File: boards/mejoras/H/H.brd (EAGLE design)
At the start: 100 x 35 mm, 37 parts, among them IC1 PIC18F4455_TQFP

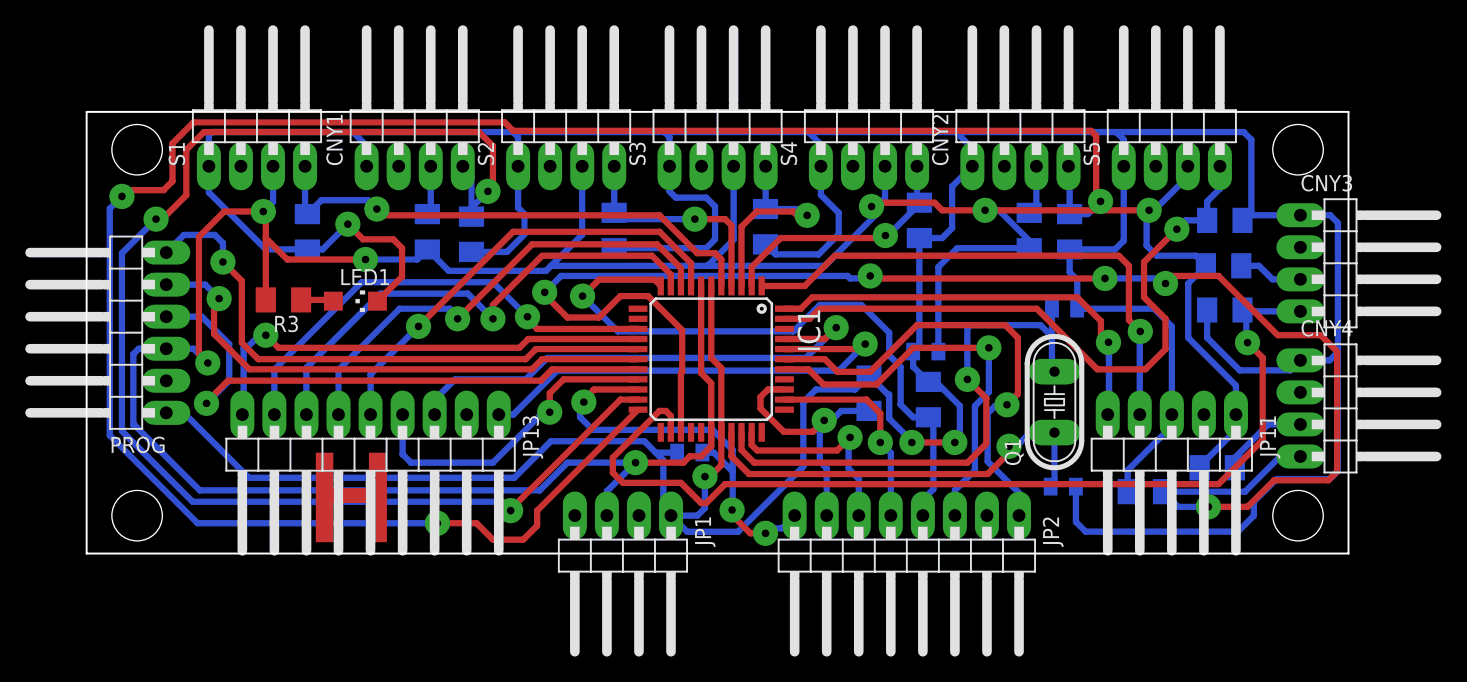
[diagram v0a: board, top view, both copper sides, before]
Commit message: updated board h and i
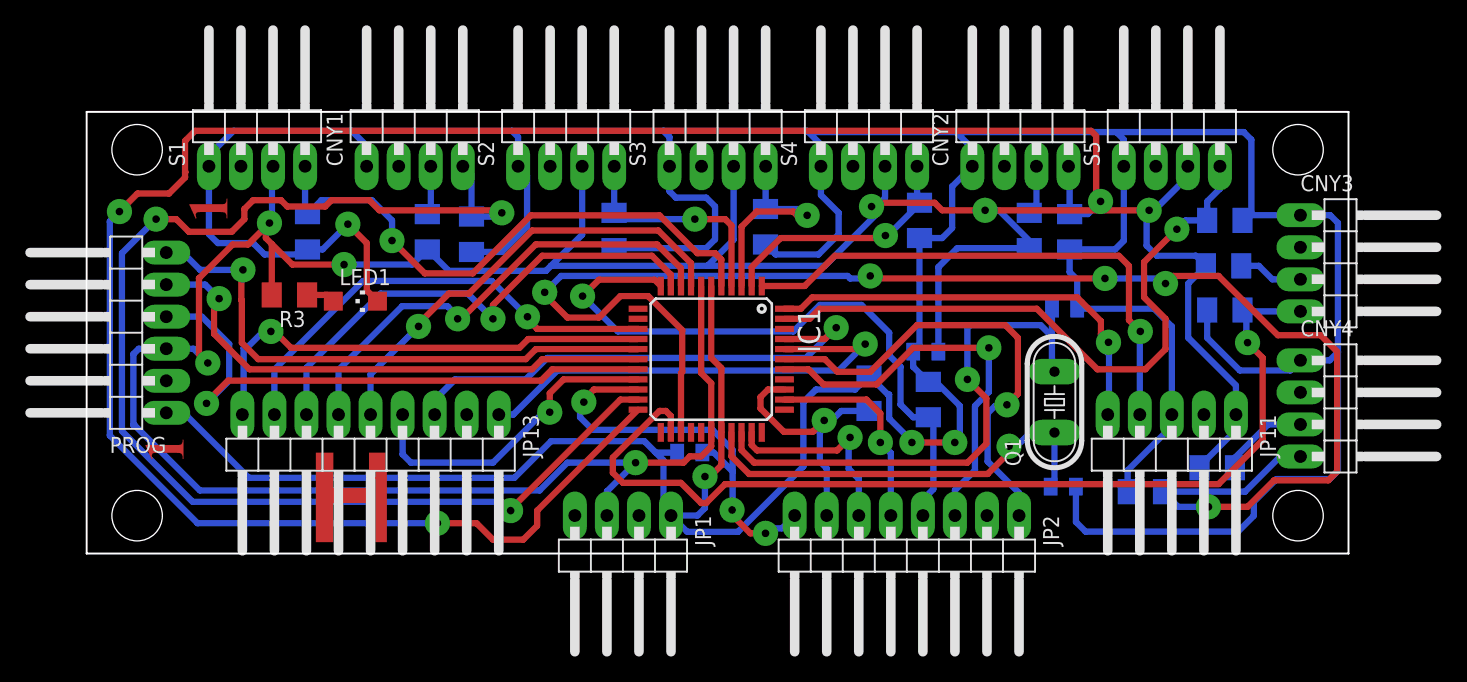
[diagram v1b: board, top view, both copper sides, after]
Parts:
- moved R3 0.61 mm to (16.1, 20.5)
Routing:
- net CNY1: track 107.8 -> 102.1 mm
- net S1: track 41.2 -> 45.9 mm
- net 5V: track 256.8 -> 254.4 mm
- net PGC: track 46.1 -> 44.8 mm
- net CNY2: track 163.5 -> 162.3 mm
- net GND: track 417.6 -> 416.7 mm
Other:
- board text added: "C:/Users/Ariel/GitHub/Sumo-Robot-Programs-Database/boards/mejoras/I/1.bmp"

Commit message: small fixes to h
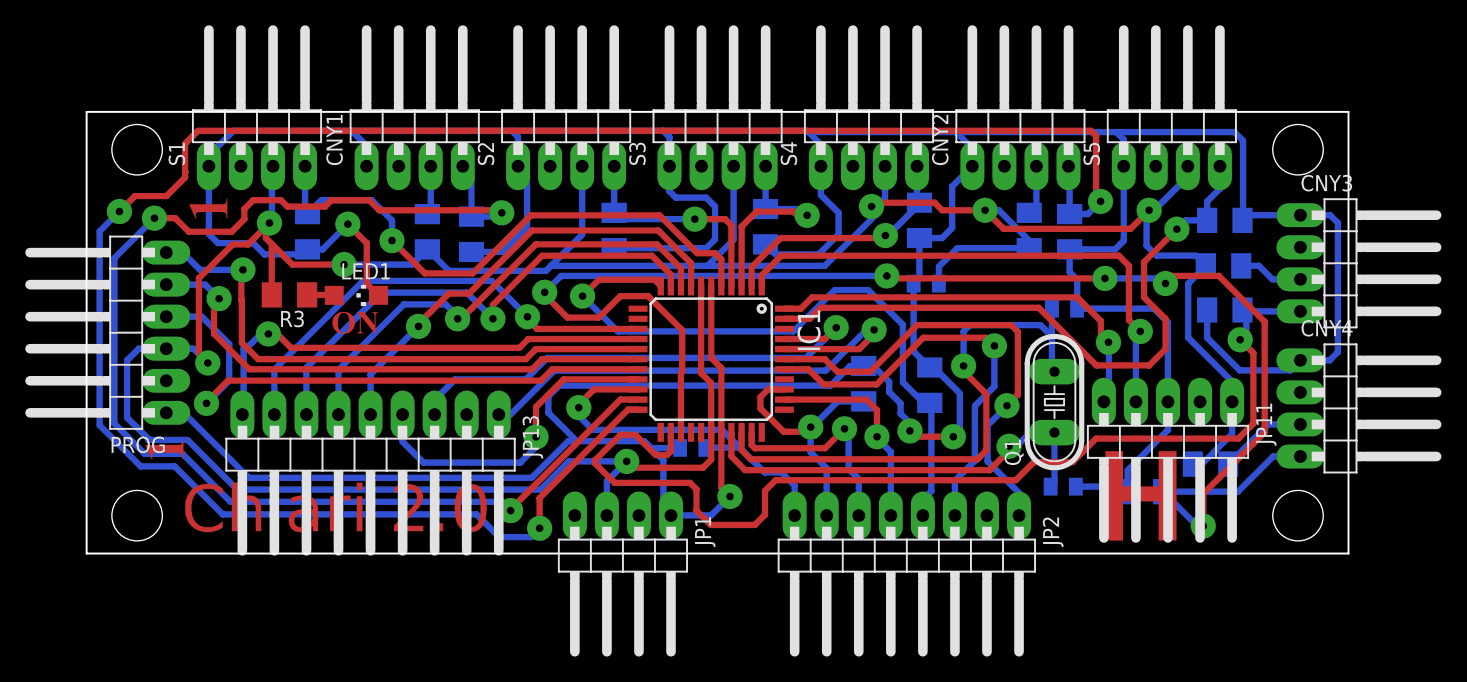
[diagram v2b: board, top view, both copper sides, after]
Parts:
- moved C3 5.39 mm to (66.5, 21.4)
- moved R1 1.15 mm to (66.8, 13.3)
- moved JP11 1.06 mm to (85.7, 8.22)
- moved R2 0.87 mm to (61.6, 13.5)
- moved R16 0.60 mm to (89.1, 7.08)
- moved LED1 0.46 mm to (21.4, 20.5)
- moved C4 0.43 mm to (48.0, 8.36)
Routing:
- net GND: track 416.7 -> 391.0 mm
- net CNY4: track 126.3 -> 117.0 mm
- net CNY3: track 79.0 -> 83.4 mm
- net VPOWER_SENSE: track 33.7 -> 30.6 mm, vias 3 -> 1
- net 5V: track 254.4 -> 251.5 mm
- net B1: track 37.9 -> 40.5 mm
- net PWM1: track 51.8 -> 53.2 mm
- net IN1B: track 32.3 -> 33.7 mm
- net CNY2: track 162.3 -> 163.4 mm
- net TX: track 34.2 -> 33.3 mm
- net CNY1: track 102.1 -> 102.8 mm
- net IN2B: track 16.0 -> 16.6 mm
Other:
- board text added: "C:/Users/Ariel/GitHub/Sumo-Robot-Programs-Database/boards/mejoras/I/ON.bmp"
- board text added: "C:/Users/Ariel/GitHub/Sumo-Robot-Programs-Database/boards/mejoras/I/chiari.bmp"
